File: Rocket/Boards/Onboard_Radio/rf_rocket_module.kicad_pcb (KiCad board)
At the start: 4 copper layers, 65.2 x 46.1 mm, 78 parts, among them J10 M80-5301042, J3 USB_B_Micro, J4 SWD JST PH, J5 Conn_01x08, J6 RFIO SMA, J7 CAN1_T, J8 CAN2_T, J9 M80-5301042, U1 TCAN1046, U2 SX1262, U3 PE4259 RF Switch, U4 STM32H562RGT6, Y1 32.000MHz, Y2 12MHz

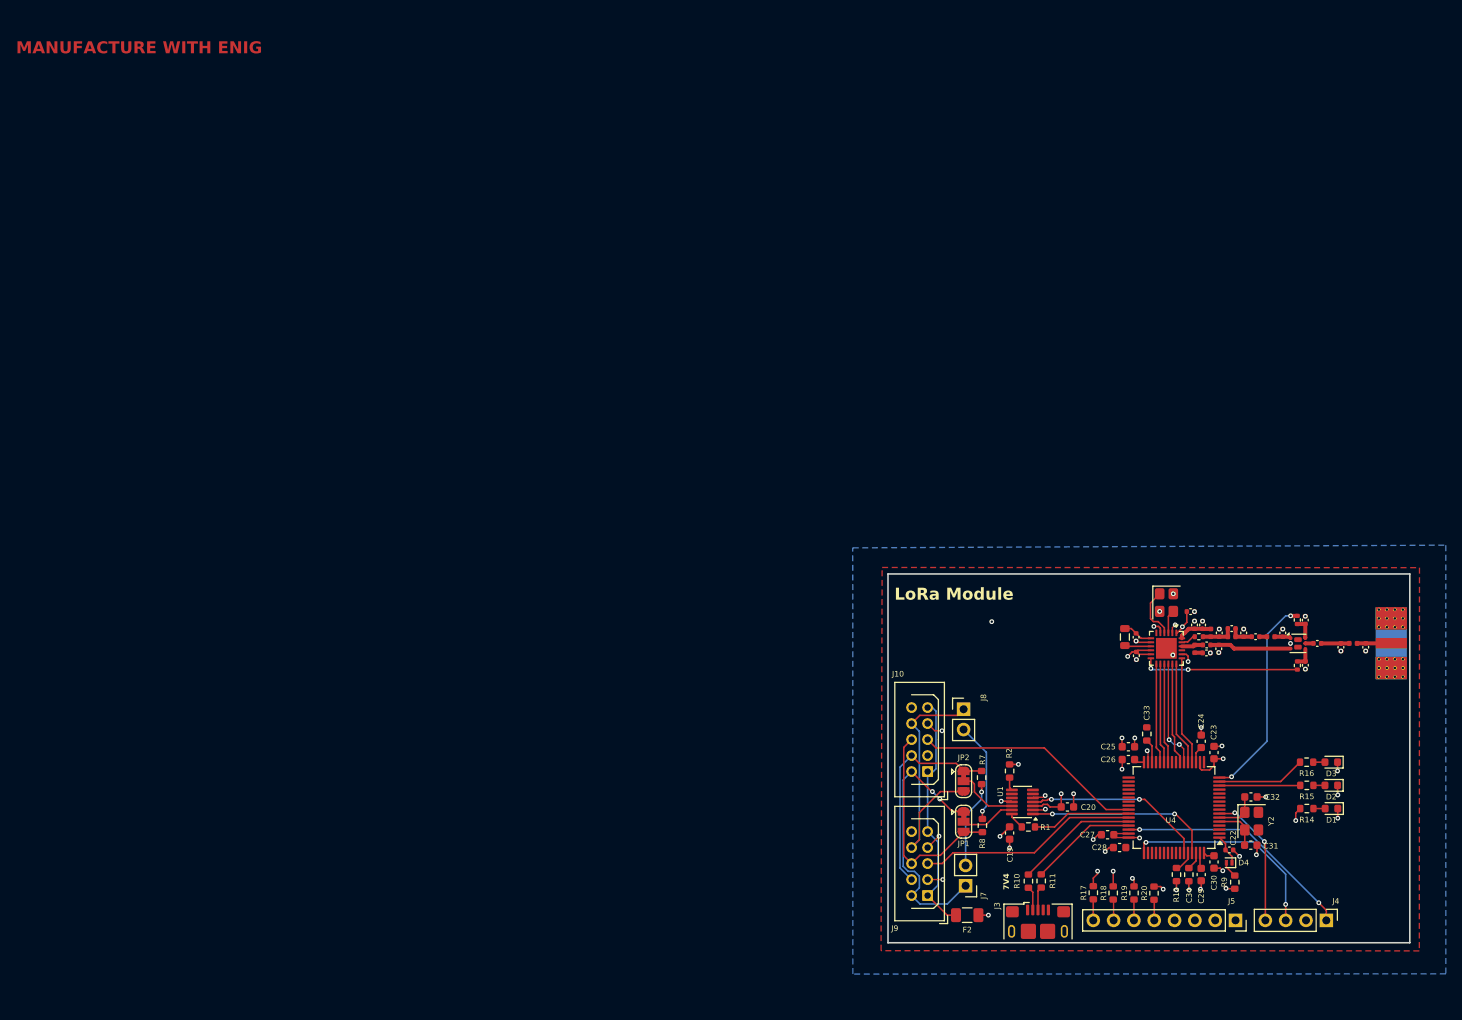
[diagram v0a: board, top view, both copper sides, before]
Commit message: pcb updates
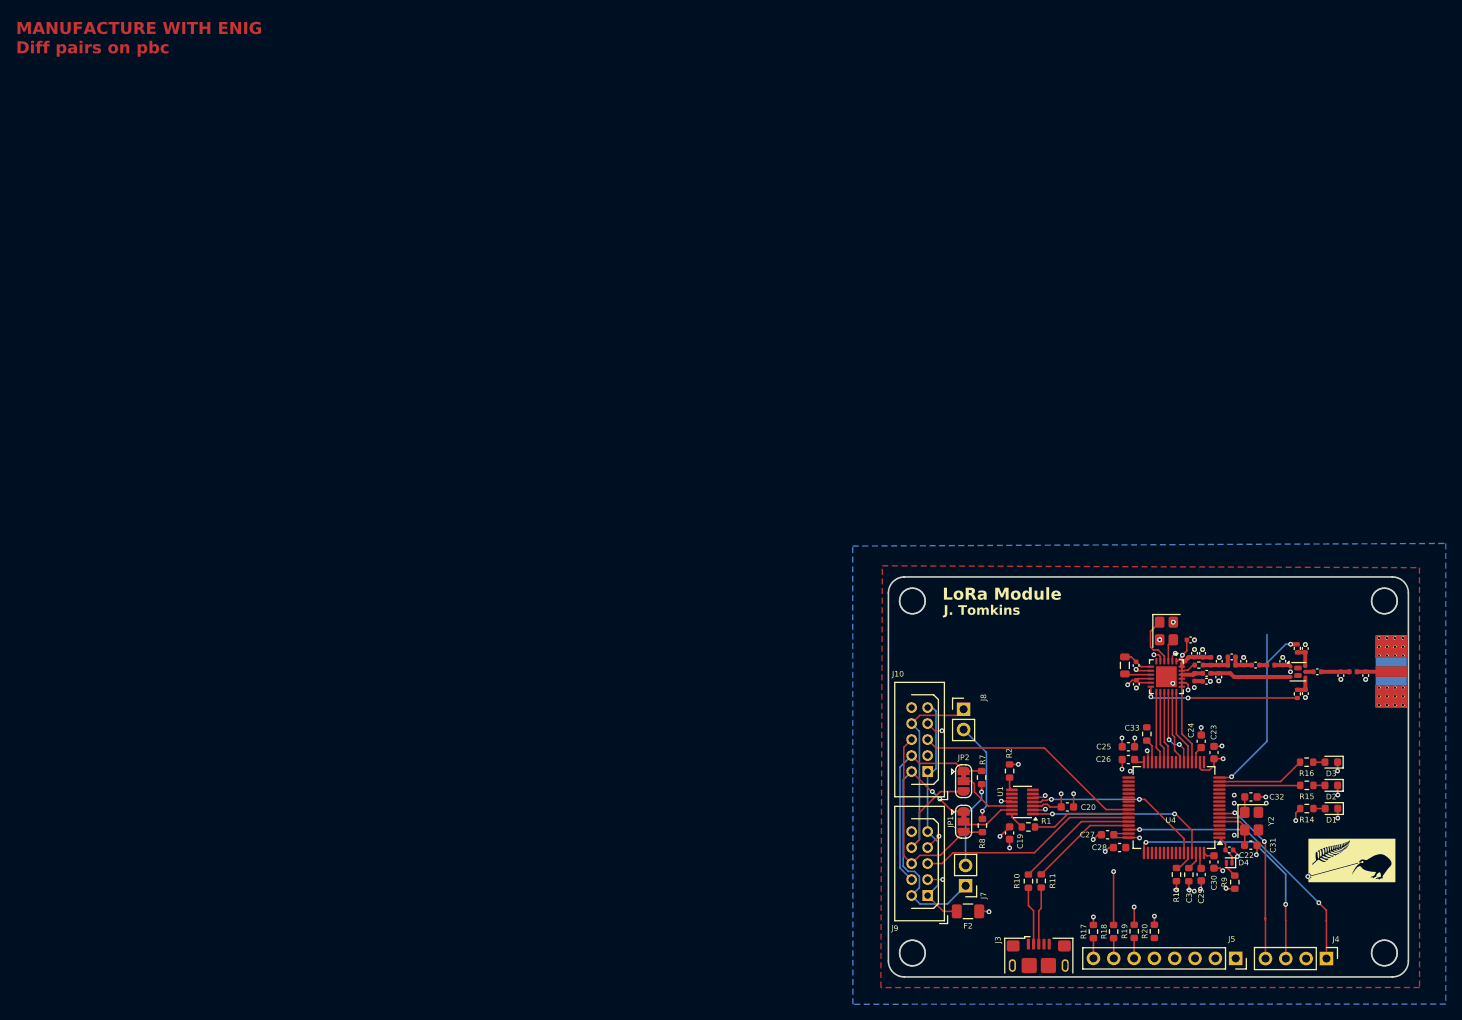
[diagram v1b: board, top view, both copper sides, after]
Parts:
- added H1: MountingHole, MountingHole:MountingHole_3.2mm_M3, F.Cu at (127.5, 86.3)
- added H2: MountingHole, MountingHole:MountingHole_3.2mm_M3, F.Cu at (127.5, 130.3)
- added H3: MountingHole, MountingHole:MountingHole_3.2mm_M3, F.Cu at (186.6, 86.3)
- added H4: MountingHole, MountingHole:MountingHole_3.2mm_M3, F.Cu at (186.6, 130.3)
- J10, J9: value M80-5301042 -> M80
- moved R17 4.85 mm to (150.2, 127.6)
- moved R18 4.83 mm to (152.7, 127.6)
- moved R19 4.80 mm to (155.3, 127.6)
- moved R20 4.78 mm to (157.8, 127.6)
- moved J4 4.78 mm to (179.3, 131.0)
- moved J5 4.75 mm to (168.0, 130.9)
- moved J3 4.27 mm to (143.3, 131.8)
- moved C1 3.55 mm to (162.8, 92.8)
- moved C10 3.55 mm to (184.2, 95.6)
- moved C12 3.55 mm to (164.3, 96.3)
- moved C13 3.55 mm to (165.8, 95.8)
- moved C14 3.55 mm to (176.7, 92.2)
- moved C16 3.55 mm to (162.3, 91.2)
- moved C17 3.55 mm to (155.5, 94.4)
- moved C2 3.55 mm to (163.8, 92.8)
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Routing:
- net /MCU/NRST: track 17.1 -> 22.1 mm
- net /MCU/SWCLK: track 30.2 -> 34.9 mm
- net /MCU/SWDIO: track 26.4 -> 31.2 mm
- net /MCU/USB_D-: track 3.00 -> 7.31 mm
- net /MCU/USB_D+: track 2.97 -> 7.19 mm
- net +7V4: track 52.7 -> 49.1 mm
- net /LoRav2/SX_NRESET: track 12.5 -> 8.93 mm
- net /LoRav2/SCK: track 12.9 -> 9.35 mm
- net /LoRav2/MOSI: track 12.7 -> 9.14 mm
- net /LoRav2/MISO: track 13.5 -> 9.95 mm
- net /LoRav2/DIO1: track 12.5 -> 8.93 mm
- net /LoRav2/BUSY: track 12.5 -> 8.93 mm
- net +5V: track 28.1 -> 31.0 mm
- net /Power Input/+7V4: track 2.59 -> 0.00 mm
- net VDD_RADIO: track 47.1 -> 48.3 mm
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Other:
- board size 65.2 x 46.1 mm -> 65 x 50 mm
- board text added: "MANUFACTURE WITH ENIG Diff pairs on pbc"
- board text removed: "7V4"
- board text removed: "MANUFACTURE WITH ENIG"
